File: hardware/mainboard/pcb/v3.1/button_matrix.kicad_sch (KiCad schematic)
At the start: 34 parts, among them U10 touch_but_square, U11 touch_but_square, U12 touch_but_square, U13 touch_but_square, U14 touch_but_square, U15 touch_but_square, U16 touch_but_square, U17 BU4551BF-E2, U18 BU4551BF-E2, U19 touch_but_square, U20 touch_but_square, U21 touch_but_square, U22 touch_but_square, U23 touch_but_square, U24 touch_but_square, U25 touch_but_square, U26 touch_but_square, U9 touch_but_square

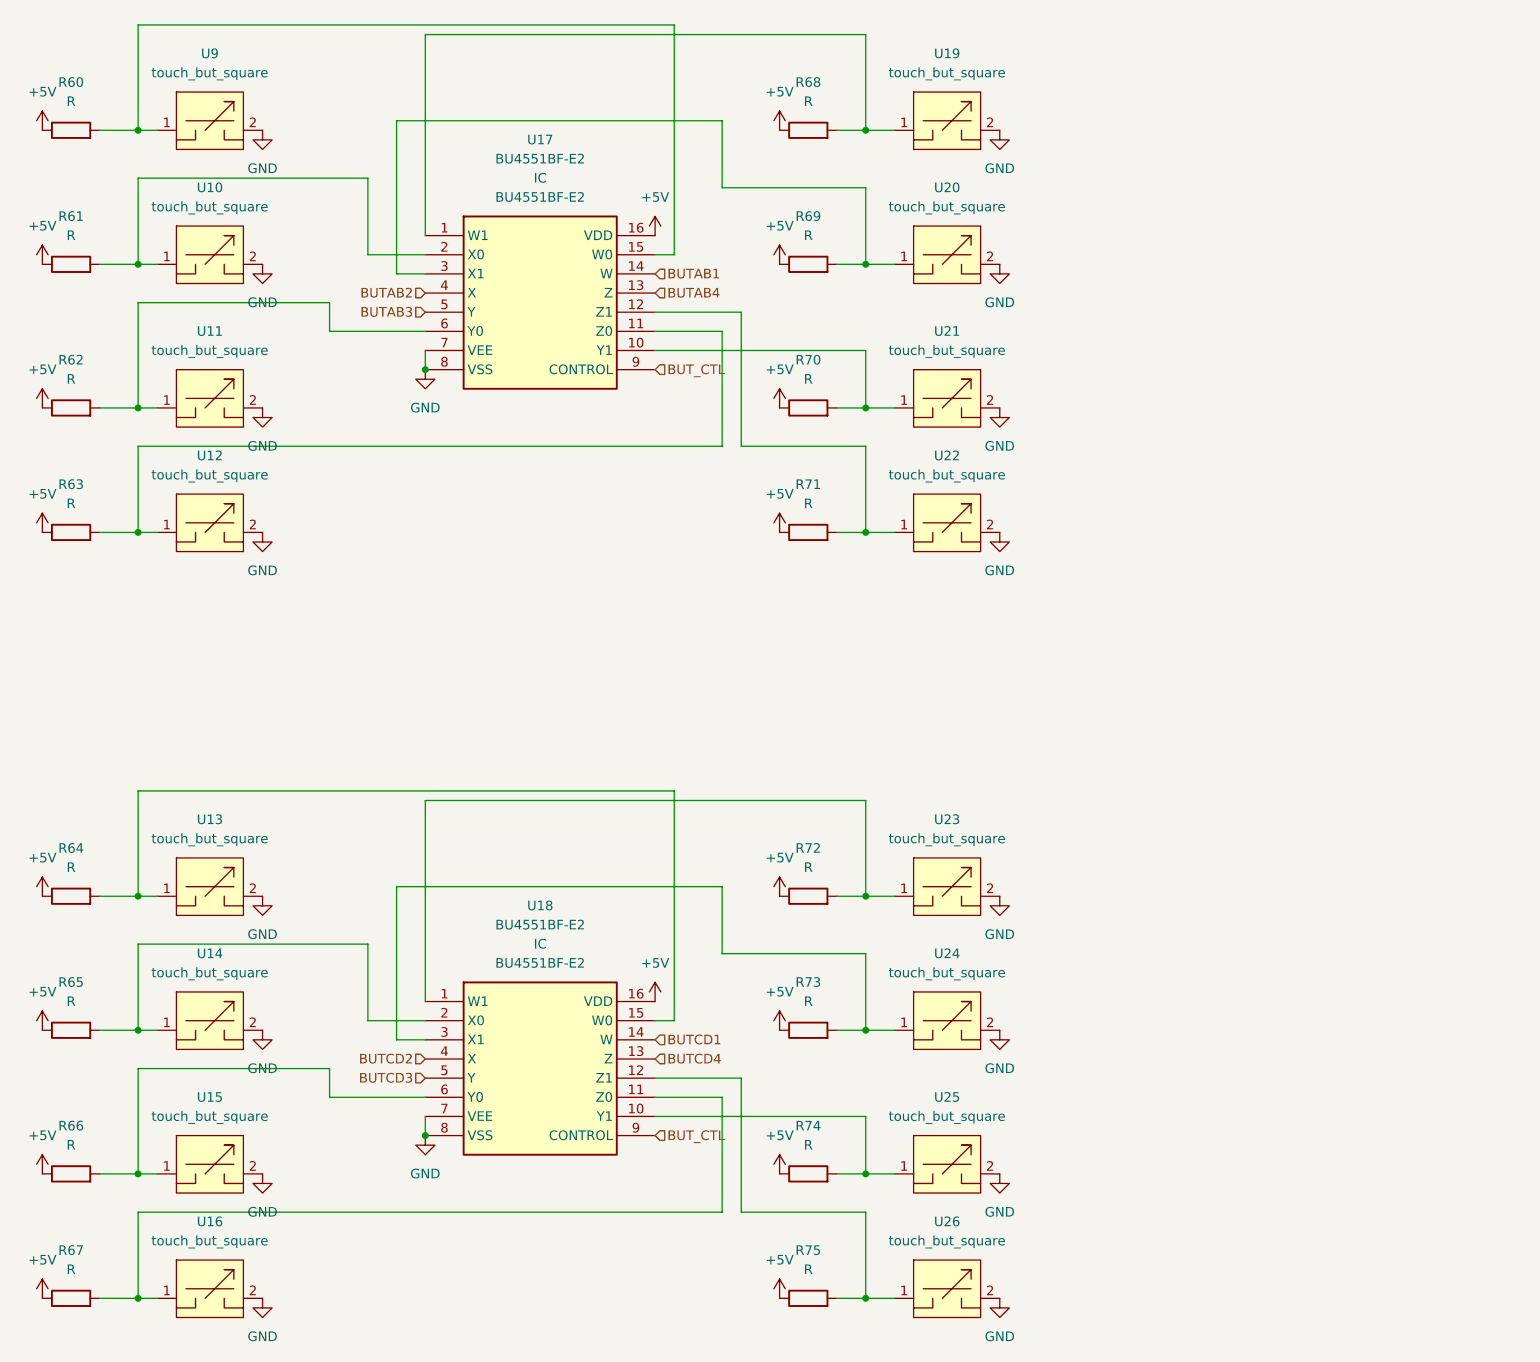
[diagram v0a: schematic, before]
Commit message: .
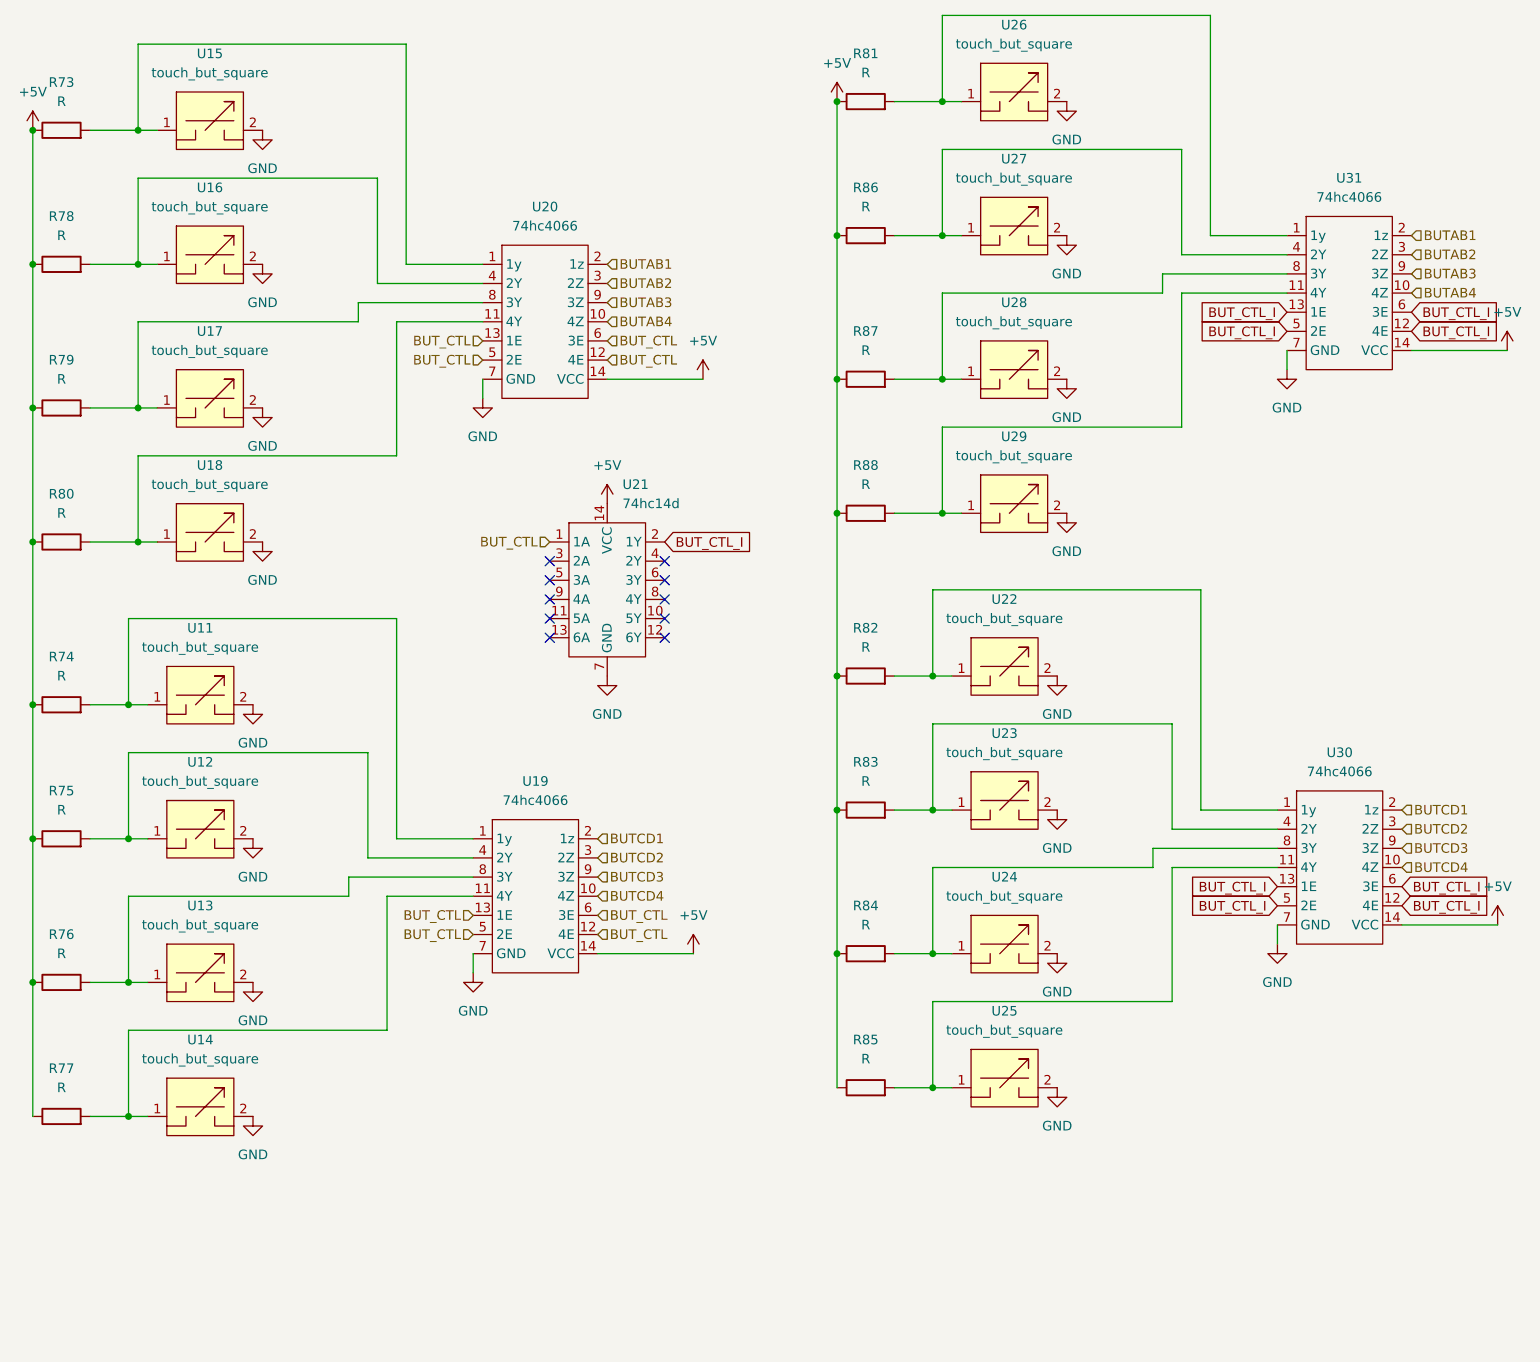
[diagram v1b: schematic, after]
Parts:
- removed R64, R65, R66, R67, R68, R69, R70, R71, R72, R73: R, Resistor_SMD:R_1206_3216Metric_Pad1.30x1.75mm_HandSolder, symbol Device:R
- removed U15, U16, U19, U20, U21: touch_but_square, 3dAudioFoot:But_Velo_Rec_1, symbol 3dAudioSym:touch_but_square
- removed U17, U18: BU4551BF-E2, 3dAudioFoot:SOIC127P620X171-16N, symbol 3dAudioSym:BU4551BF-E2
- added R76, R77, R81, R82, R83, R84, R85, R86, R87, R88: R, Resistor_SMD:R_1206_3216Metric_Pad1.30x1.75mm_HandSolder, symbol Device:R
- added U11, U12, U27, U28, U29: touch_but_square, 3dAudioFoot:But_Velo_Rec_1, symbol 3dAudioSym:touch_but_square
- added U19, U20, U30, U31: 74hc4066, Package_SO:SOIC-14_3.9x8.7mm_P1.27mm, symbol 3dAudioSym:74hc4066
- added U21: 74hc14d, Package_SO:SOIC-14_3.9x8.7mm_P1.27mm, symbol 3dAudioSym:74hc14d
- renumbered R60 to R73, R61 to R78, R62 to R79, R63 to R80, U9 to U15, U10 to U16, U11 to U17, U12 to U18
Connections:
- net +5V: now also R76.1, R77.1, R81.1, R82.1, R83.1, R84.1, R85.1, R86.1, R87.1, R88.1, U19.14 (VCC), U20.14 (VCC), U21.14 (VCC), U30.14 (VCC), U31.14 (VCC)
- net BUTAB1: now also U20.2 (1z), U31.2 (1z)
- net BUTAB2: now also U20.3 (2Z), U31.3 (2Z)
- net BUTAB3: now also U20.9 (3Z), U31.9 (3Z)
- net BUTAB4: now also U20.10 (4Z), U31.10 (4Z)
- net BUTCD1: now also U19.2 (1z), U30.2 (1z)
- net BUTCD2: now also U19.3 (2Z), U30.3 (2Z)
- net BUTCD3: now also U19.9 (3Z), U30.9 (3Z)
- net BUTCD4: now also U19.10 (4Z), U30.10 (4Z)
- net BUT_CTL: now also U19.12 (4E), U19.13 (1E), U19.5 (2E), U19.6 (3E), U20.12 (4E), U20.13 (1E), U20.5 (2E), U20.6 (3E), U21.1 (1A)
- net GND: now also U11.2, U12.2, U19.7 (GND), U20.7 (GND), U21.7 (GND), U27.2, U28.2, U29.2, U30.7 (GND), U31.7 (GND)
- net at U25.1: now also R85.2, U30.11 (4Y); no longer R74.2
- net at U23.1: now also R83.2, U30.4 (2Y)
- net at U22.1: now also R82.2, U30.1 (1y)
- net at U13.1: now also R76.2, U19.8 (3Y)
- net at R73.2, U15.1: now also U20.1 (1y)
- net at R80.2, U18.1: now also U20.11 (4Y)
- net at R79.2, U17.1: now also U20.8 (3Y)
- net at R78.2, U16.1: now also U20.4 (2Y)
- net at R75.2: now also U12.1, U19.4 (2Y); no longer U26.1
- net at U14.1: now also R77.2, U19.11 (4Y)
- net at U24.1: now also R84.2, U30.8 (3Y)
- new net: R88.2, U29.1, U31.11 (4Y)
- new net: R87.2, U28.1, U31.8 (3Y)
- new net: R86.2, U27.1, U31.4 (2Y)
- new net: R81.2, U26.1, U31.1 (1y)
- new net: R74.2, U11.1, U19.1 (1y)
- new net BUT_CTL_I: U21.2 (1Y), U30.12 (4E), U30.13 (1E), U30.5 (2E), U30.6 (3E), U31.12 (4E), U31.13 (1E), U31.5 (2E), U31.6 (3E)
- no-connect marks 0 -> 10
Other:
- moved on the sheet: R73, R78, R79, R80, U18
